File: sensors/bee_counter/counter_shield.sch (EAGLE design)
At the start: 33 parts

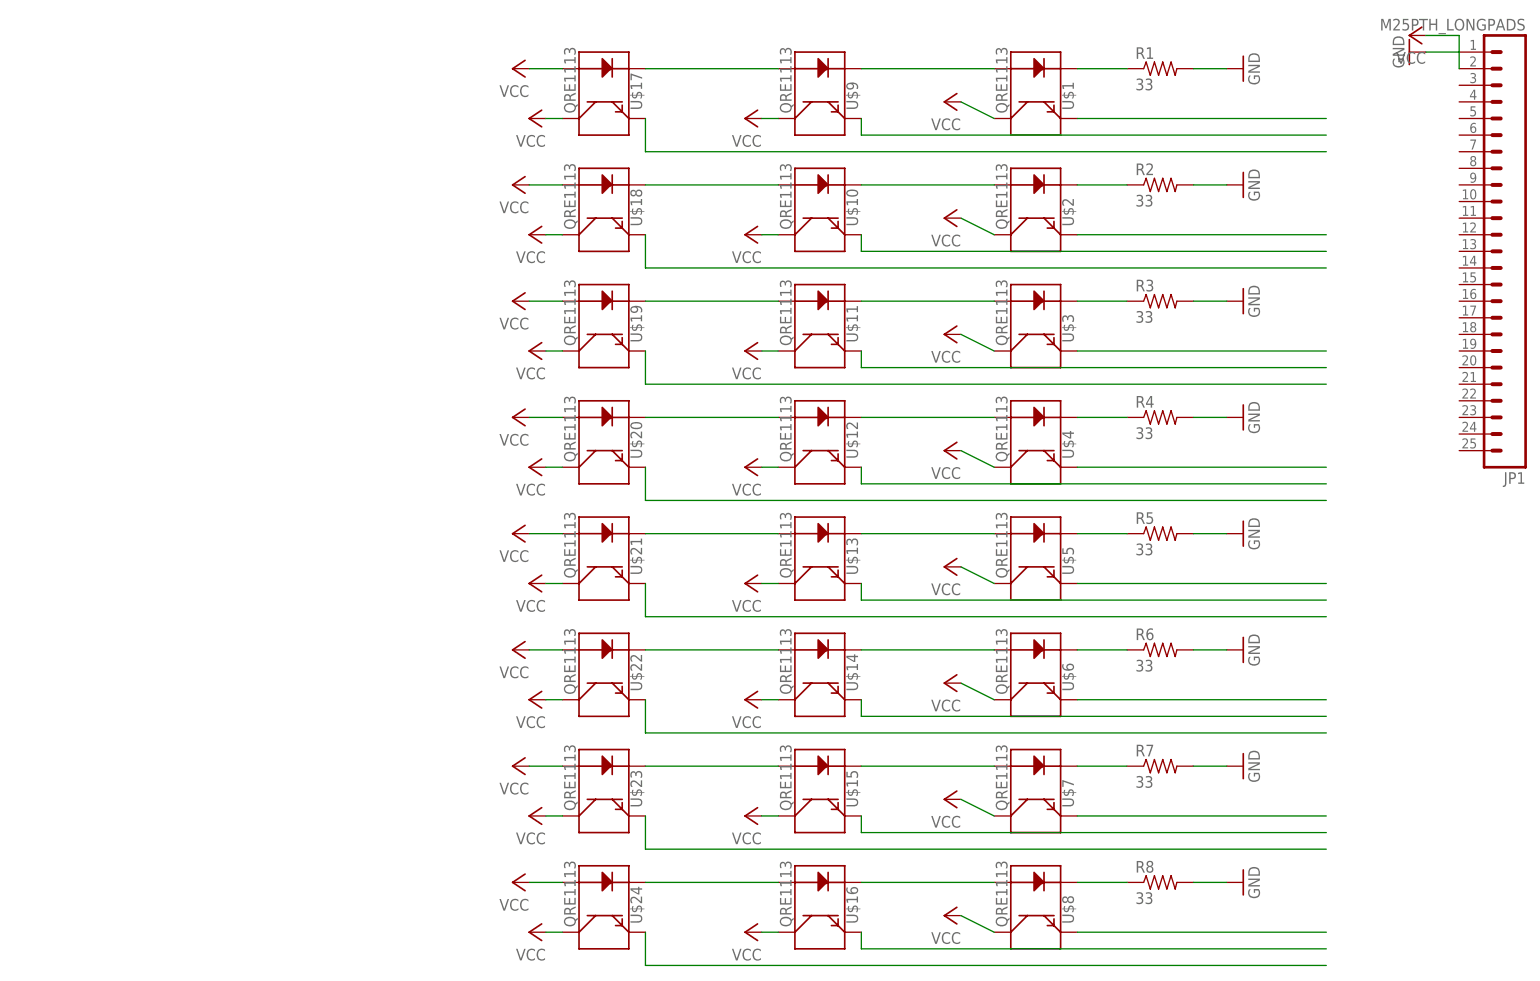
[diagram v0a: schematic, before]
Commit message: laser stuff
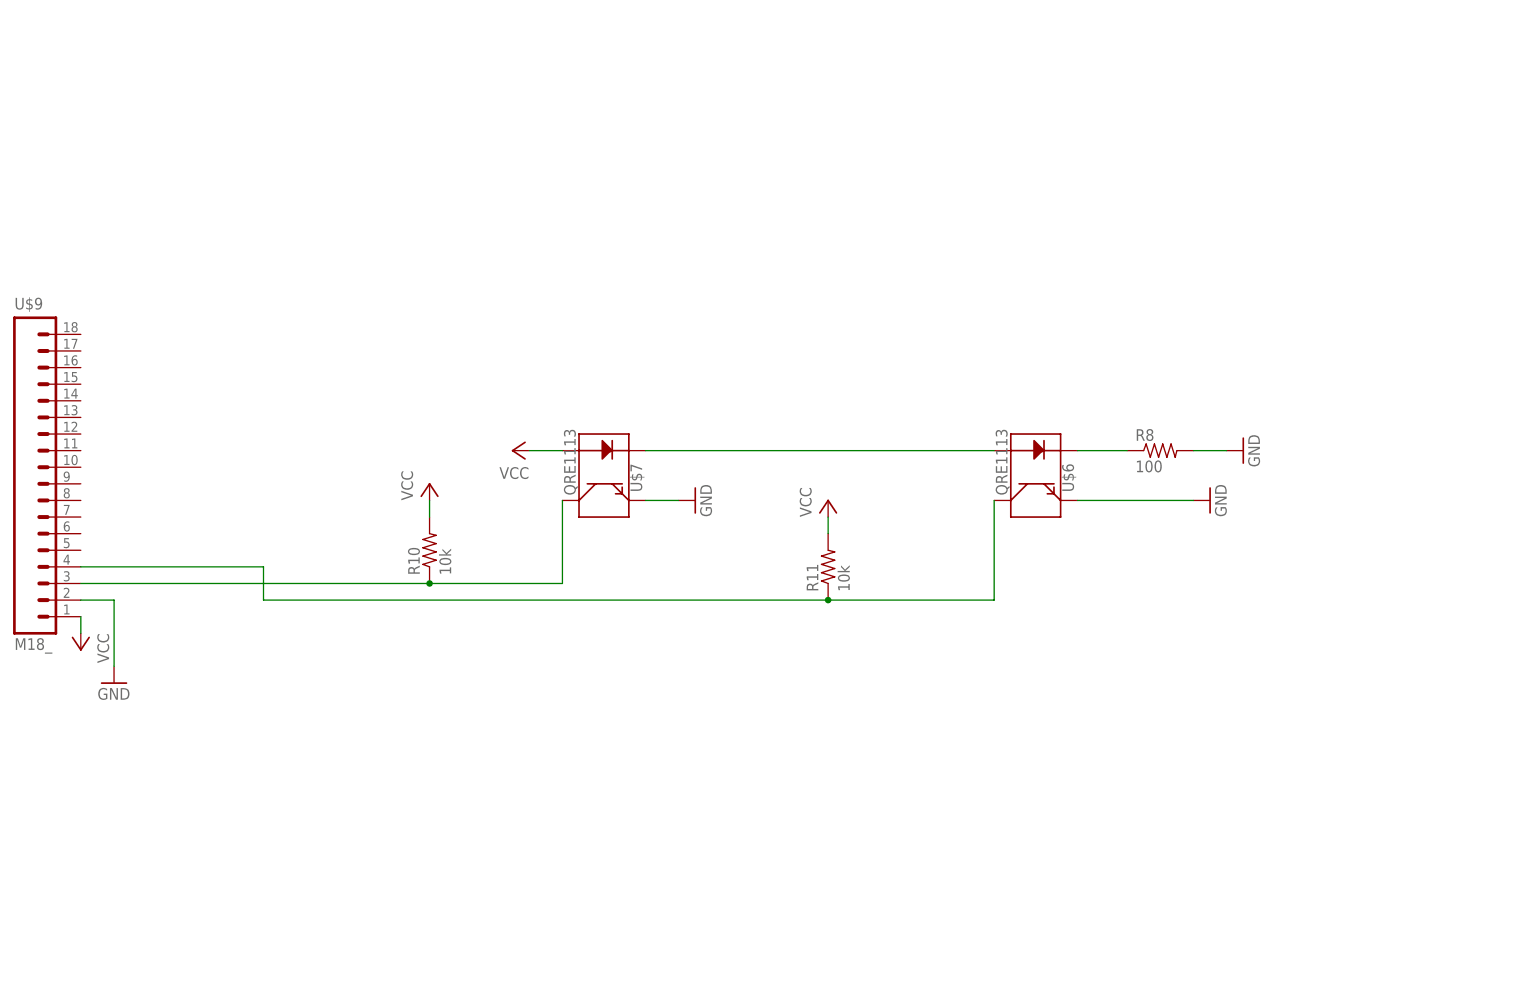
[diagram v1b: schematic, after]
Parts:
- removed JP1: M25PTH_LONGPADS, SparkFun-Connectors:M25PTH_LONGPADS
- removed R1, R2, R3, R4, R5, R6, R7: 33, 01_ng:RESISTOR1206
- removed U$1, U$10, U$11, U$12, U$13, U$14, U$15, U$16, U$17, U$18, U$19, U$2, U$20, U$21, U$22, U$23, U$24, U$3, U$4, U$5, U$8: QRE1113, SparkFun-Sensors:QRE1113
- added R10, R11: 10k, 01_ng:RESISTOR1206
- R8: value 33 -> 100
- U$9: value QRE1113 -> M18_; device SparkFun-Sensors:QRE1113 -> SparkFun-Connectors:M18_
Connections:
- removed net N$1: U$17.K, U$9.A
- removed net N$14: U$15.K, U$7.A
- removed net N$15: U$16.K, U$8.A
- removed net N$16: U$16.A, U$24.K
- removed net N$17: R8.1, U$8.K
- removed net N$18: R7.1, U$7.K
- removed net N$19: R6.1, U$6.K
- removed net N$2: U$1.A, U$9.K
- removed net N$20: R5.1, U$5.K
- removed net N$21: R4.1, U$4.K
- removed net N$22: R3.1, U$3.K
- removed net N$23: R2.1, U$2.K
- removed net N$24: R1.1, U$1.K
- removed net N$25: U$17.E
- removed net N$26: U$9.E
- removed net N$27: U$1.E
- removed net N$28: U$18.E
- removed net N$29: U$10.E
- removed net N$3: U$10.A, U$18.K
- removed net N$30: U$2.E
- removed net N$31: U$19.E
- removed net N$32: U$11.E
- removed net N$33: U$3.E
- removed net N$34: U$20.E
- removed net N$35: U$12.E
- removed net N$36: U$4.E
- removed net N$37: U$21.E
- removed net N$38: U$13.E
- removed net N$39: U$5.E
- removed net N$4: U$10.K, U$2.A
- removed net N$40: U$22.E
- removed net N$41: U$14.E
- removed net N$42: U$6.E
- removed net N$43: U$23.E
- removed net N$44: U$15.E
- removed net N$45: U$7.E
- removed net N$46: U$24.E
- removed net N$47: U$16.E
- removed net N$48: U$8.E
- removed net N$5: U$11.K, U$3.A
- removed net N$6: U$11.A, U$19.K
- removed net N$7: U$12.A, U$20.K
- removed net N$8: U$12.K, U$4.A
- removed net N$9: U$13.A, U$21.K
- net GND: now also U$6.E, U$7.E, U$9.2; no longer JP1.2, R1.2, R2.2, R3.2, R4.2, R5.2, R6.2, R7.2
- net N$10: now also R8.1, U$6.K; no longer U$13.K, U$5.A
- net N$11: now also U$7.K; no longer U$14.K
- net N$12: now also R10.1, U$7.C, U$9.3; no longer U$14.A, U$22.K
- net N$13: now also R11.1, U$6.C, U$9.4; no longer U$15.A, U$23.K
- net VCC: now also R10.2, R11.2, U$7.A, U$9.1; no longer JP1.1, U$1.C, U$10.C, U$11.C, U$12.C, U$13.C, U$14.C, U$15.C, U$16.C, U$17.A, U$17.C, U$18.A, U$18.C, U$19.A, U$19.C, U$2.C, U$20.A, U$20.C, U$21.A, U$21.C, U$22.A, U$22.C, U$23.A, U$23.C, U$24.A, U$24.C, U$3.C, U$4.C, U$5.C, U$6.C, U$7.C, U$8.C, U$9.C
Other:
- moved on the sheet: R8, U$6, U$7
